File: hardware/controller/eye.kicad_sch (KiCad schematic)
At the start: 25 parts, among them U4 baochip1x, U5 EMS4000RSW, Y1 48 MHz

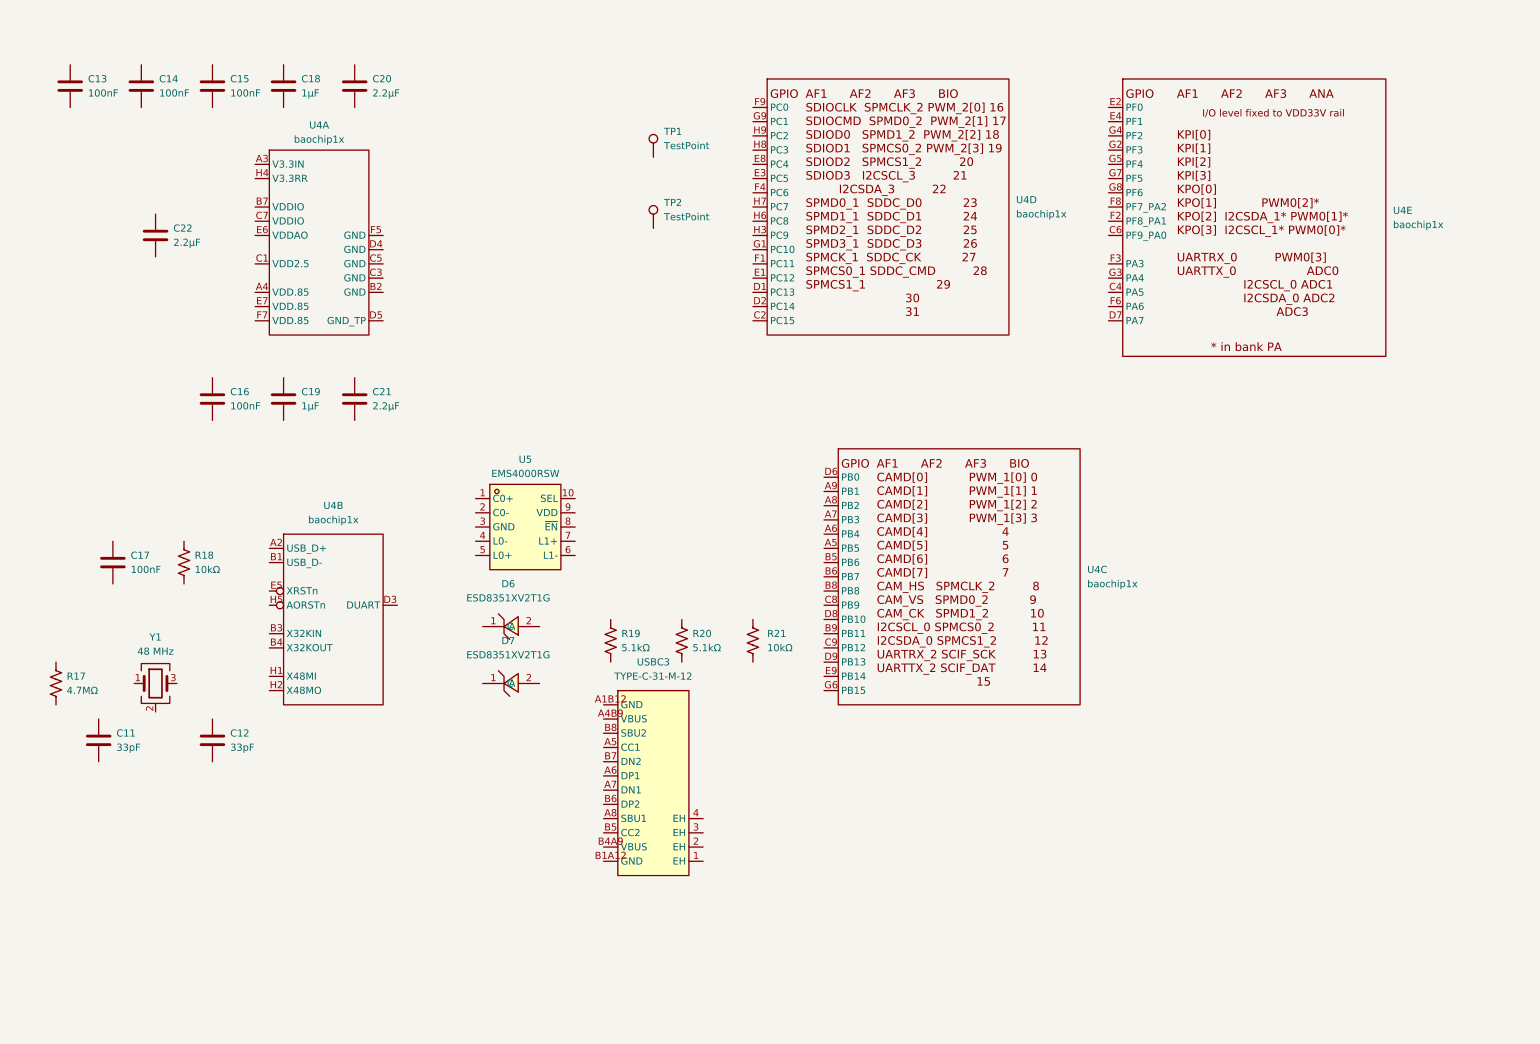
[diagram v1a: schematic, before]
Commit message: more schematic work
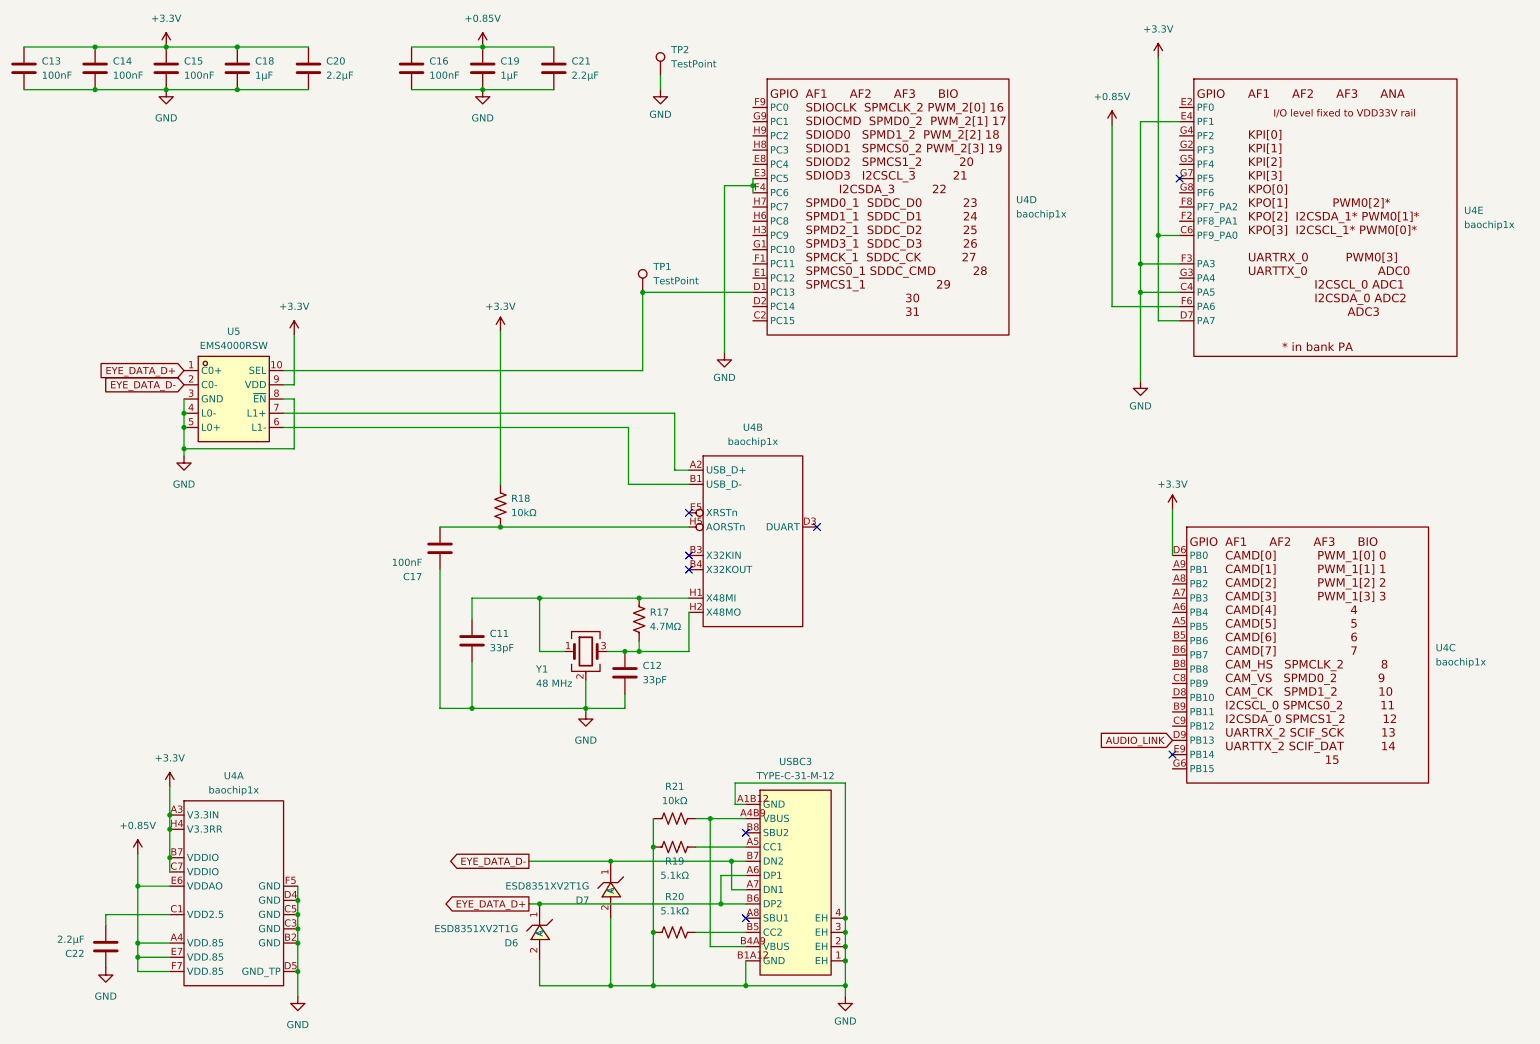
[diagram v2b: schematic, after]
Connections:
- net at C12.1: now also R17.2, U4.H2 (X48MO), Y1.3
- net GND: now reaches C12.2
- net GND: now also C11.2, C13.2, C14.2, C15.2, C16.2, C17.2, C18.2, C19.2, C20.2, C21.2, C22.2, D6.2 (A), D7.2 (A), R19.1, R20.1, R21.1, TP2.1, U4.B2 (GND), U4.C3 (GND), U4.C4 (PA5), U4.C5 (GND), U4.D4 (GND), U4.D5 (GND_TP), U4.E3 (PC5), U4.E4 (PF1), U4.F3 (PA3), U4.F4 (PC6), U4.F5 (GND), U5.3 (GND), U5.4 (L0-), U5.5 (L0+), U5.8 (~{EN}), USBC3.1 (EH), USBC3.2 (EH), USBC3.3 (EH), USBC3.4 (EH), USBC3.A1B12 (GND), USBC3.B1A12 (GND), Y1.2 (G), Y1.4 (G)
- net +3.3V: now reaches C15.1
- net +3.3V: now also C13.1, C14.1, C18.1, C20.1, R18.1, U4.A3 (V3.3IN), U4.B7 (VDDIO), U4.C6 (PF9_PA0), U4.C7 (VDDIO), U4.D6 (PB0), U4.D7 (PA7), U4.H4 (V3.3RR), U5.9 (VDD)
- net at U4.D1 (PC13): now also TP1.1, U5.10 (SEL)
- net at R19.2: now also USBC3.A5 (CC1)
- net +0.85V: now reaches U4.A4 (VDD.85)
- net +0.85V: now also C16.1, C19.1, C21.1, U4.E6 (VDDAO), U4.E7 (VDD.85), U4.F6 (PA6), U4.F7 (VDD.85)
- net at U4.C1 (VDD2.5): now also C22.1
- net at U4.A2 (USB_D+): now also U5.7 (L1+)
- net at U4.B1 (USB_D-): now also U5.6 (L1-)
- net at U4.H1 (X48MI): now also C11.1, R17.1, Y1.1
- net at U4.H5 (AORSTn): now also C17.1, R18.2
- net EYE_DATA_D-: now reaches D7.1 (C)
- net EYE_DATA_D-: now also U5.2 (C0-), USBC3.A7 (DN1), USBC3.B7 (DN2)
- net EYE_DATA_D+: now reaches U5.1 (C0+)
- net EYE_DATA_D+: now also D6.1 (C), USBC3.A6 (DP1), USBC3.B6 (DP2)
- net AUDIO_LINK: now reaches U4.D9 (PB13)
- net at R21.2: now also USBC3.A4B9 (VBUS), USBC3.B4A9 (VBUS)
- net at R20.2: now also USBC3.B5 (CC2)
- no-connect marks 0 -> 8
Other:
- moved on the sheet: C11, C12, C13, C14, C15, C16, C17, C18, C19, C20, C21, C22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
